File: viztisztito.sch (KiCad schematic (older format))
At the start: 0 parts

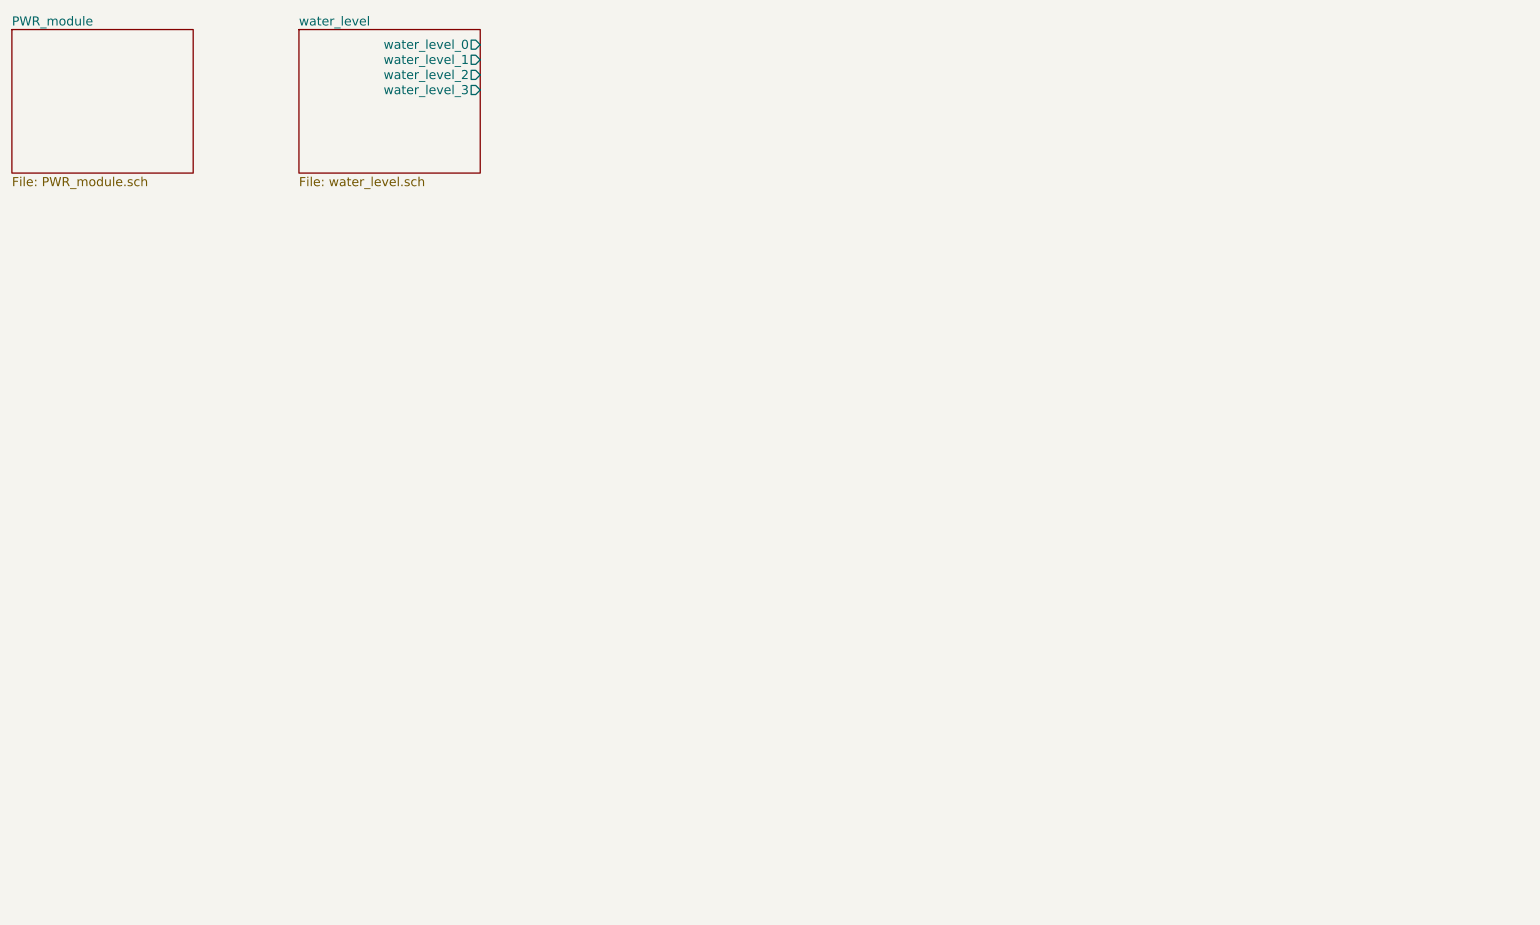
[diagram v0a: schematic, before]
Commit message: sch almost ready
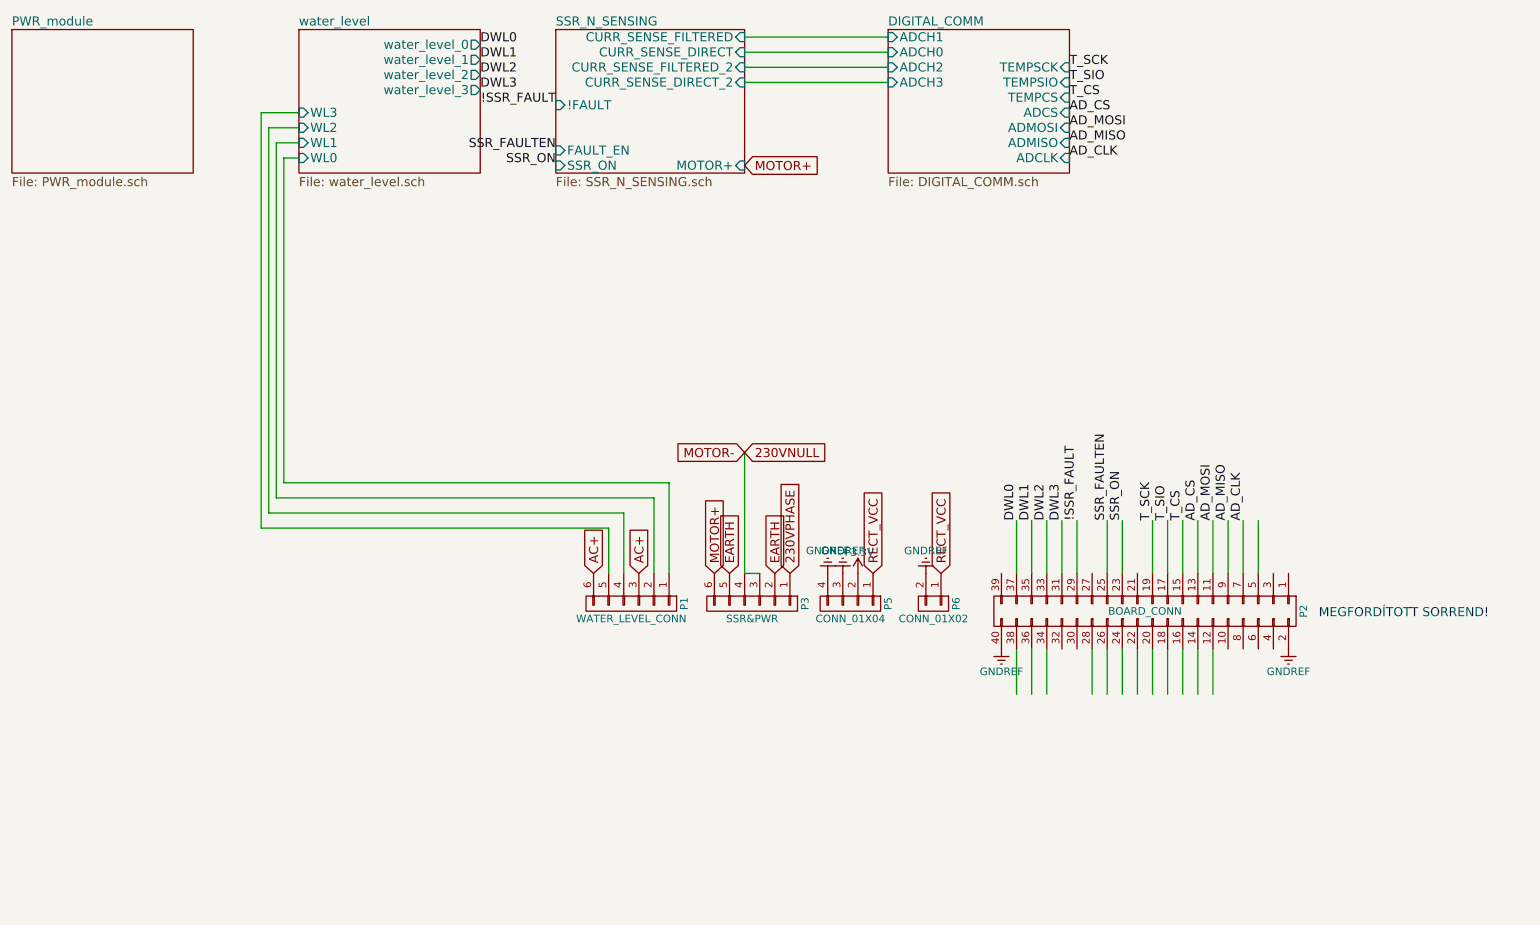
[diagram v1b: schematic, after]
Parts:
- added P1: WATER_LEVEL_CONN, symbol CONN_01X06
- added P2: BOARD_CONN, Socket_Strips:Socket_Strip_Straight_2x20, symbol CONN_02X20
- added P3: SSR&PWR, symbol CONN_01X06
- added P5: CONN_01X04, symbol CONN_01X04
- added P6: CONN_01X02, Pin_Headers:Pin_Header_Straight_1x02, symbol CONN_01X02
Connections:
- net labels added: !SSR_FAULT, +3.3V, 230VNULL, 230VPHASE, AC+, AD_CLK, AD_CS, AD_MISO, AD_MOSI, DWL0, DWL1, DWL2, DWL3, EARTH, GNDREF, MOTOR+, MOTOR-, RECT_VCC, SSR_FAULTEN, SSR_ON, T_CS, T_SCK, T_SIO
- wire segments 0 -> 49
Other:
- note added: "MEGFORDÍTOTT SORREND!"

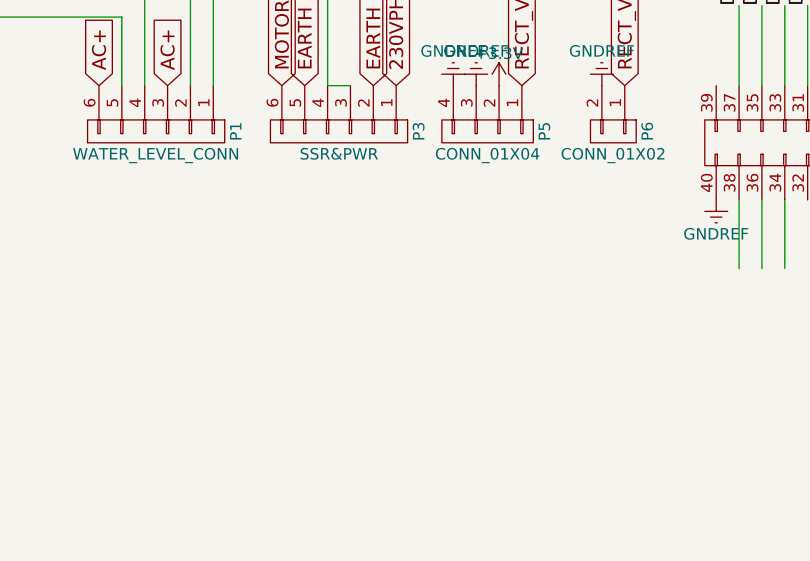
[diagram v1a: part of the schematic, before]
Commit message: sch ready, begining of layout
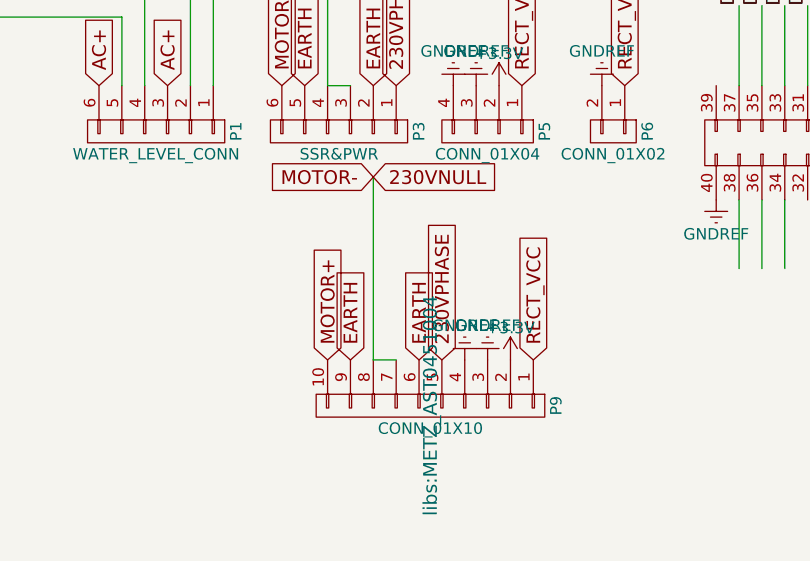
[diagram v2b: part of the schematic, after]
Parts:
- added P9: CONN_01X10, libs:METZ_AST0451004, symbol CONN_01X10
- P1, P3: footprint (none) -> libs:METZ_AST1350604
- P5: footprint (none) -> libs:METZ_AST1350404
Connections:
- wire segments 49 -> 51
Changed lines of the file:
@@
 F 0 "P1" H 5350 5150 50  0000 C CNN
 F 1 "WATER_LEVEL_CONN" V 5450 4800 50  0000 C CNN
-F 2 "" H 5350 4800 60  0001 C CNN
+F 2 "libs:METZ_AST1350604" H 5350 4800 60  0001 C CNN
 F 3 "" H 5350 4800 60  0000 C CNN
 	1    5350 4800
@@
 F 0 "P3" H 6150 5150 50  0000 C CNN
 F 1 "SSR&PWR" V 6250 4800 50  0000 C CNN
-F 2 "" H 6150 4800 60  0001 C CNN
+F 2 "libs:METZ_AST1350604" H 6150 4800 60  0001 C CNN
 F 3 "" H 6150 4800 60  0000 C CNN
 	1    6150 4800
@@
 F 0 "P5" H 6800 5050 50  0000 C CNN
 F 1 "CONN_01X04" V 6900 4800 50  0000 C CNN
-F 2 "" H 6800 4800 60  0001 C CNN
+F 2 "libs:METZ_AST1350404" H 6800 4800 60  0001 C CNN
 F 3 "" H 6800 4800 60  0000 C CNN
 	1    6800 4800
@@
 Wire Wire Line
 	6100 1350 7050 1350
+$Comp
+L CONN_01X10 P9
+U 1 1 5626D6E9
+P 6550 6000
+F 0 "P9" H 6550 6550 50  0000 C CNN
+F 1 "CONN_01X10" V 6650 6000 50  0000 C CNN
+F 2 "libs:METZ_AST0451004" H 6550 6000 60  0000 C CNN
+F 3 "" H 6550 6000 60  0000 C CNN
+	1    6550 6000
+	0    1    1    0
+$EndComp
+Text GLabel 7000 5800 1    60   Input ~ 0
+RECT_VCC
+$Comp
+L GNDREF #PWR07
+U 1 1 5626F098
+P 6700 5800
+F 0 "#PWR07" H 6700 5550 50  0001 C CNN
+F 1 "GNDREF" H 6700 5650 50  0000 C CNN
+F 2 "" H 6700 5800 60  0000 C CNN
+F 3 "" H 6700 5800 60  0000 C CNN
+	1    6700 5800
+	-1   0    0    1
+$EndComp
+$Comp
+L +3.3V #PWR08
+U 1 1 5626F09E
+P 6900 5800
+F 0 "#PWR08" H 6900 5650 50  0001 C CNN
+F 1 "+3.3V" H 6900 5940 50  0000 C CNN
+F 2 "" H 6900 5800 60  0000 C CNN
+F 3 "" H 6900 5800 60  0000 C CNN
+	1    6900 5800
+	1    0    0    -1
+$EndComp
+$Comp
+L GNDREF #PWR09
+U 1 1 5626F0A4
+P 6800 5800
+F 0 "#PWR09" H 6800 5550 50  0001 C CNN
+F 1 "GNDREF" H 6800 5650 50  0000 C CNN
+F 2 "" H 6800 5800 60  0000 C CNN
+F 3 "" H 6800 5800 60  0000 C CNN
+	1    6800 5800
+	-1   0    0    1
+$EndComp
+Text GLabel 6500 5800 1    60   Input ~ 0
+EARTH
+Text GLabel 6100 5800 1    60   Input ~ 0
+MOTOR+
+Text GLabel 6300 5000 0    60   Input ~ 0
+MOTOR-
+Text GLabel 6200 5800 1    60   Input ~ 0
+EARTH
+Wire Wire Line
+	6300 5000 6300 5800
+Wire Wire Line
+	6300 5800 6400 5800
+Text GLabel 6600 5800 1    60   Input ~ 0
+230VPHASE
+Text GLabel 6300 5000 2    60   Input ~ 0
+230VNULL
 $EndSCHEMATC

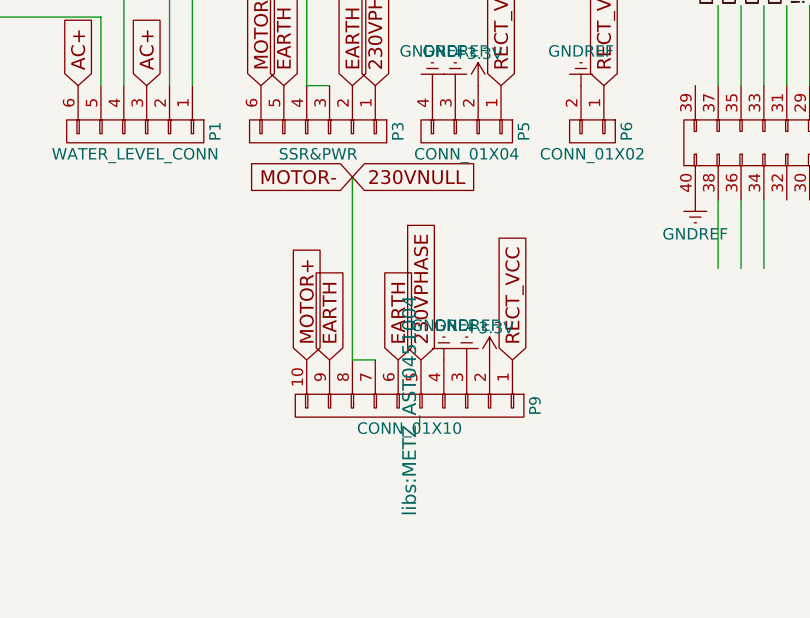
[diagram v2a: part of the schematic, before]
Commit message: layout beginning
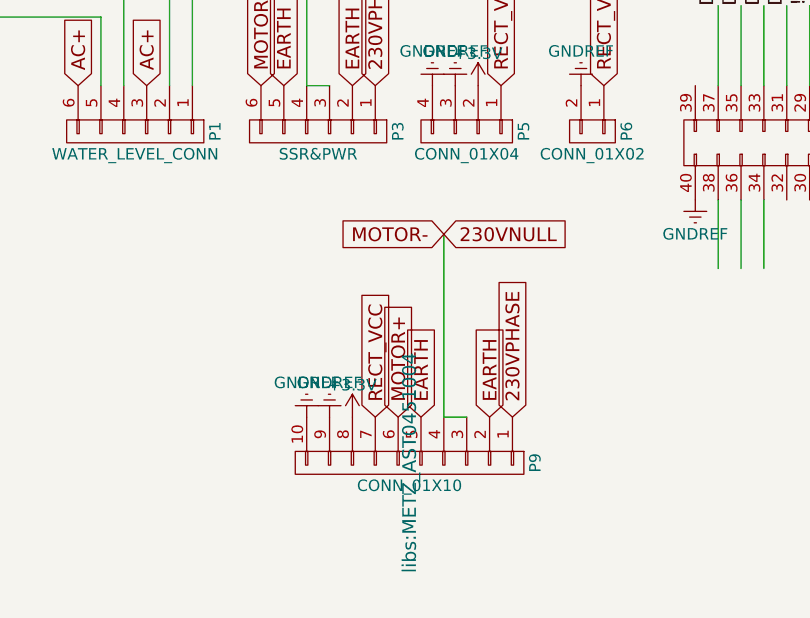
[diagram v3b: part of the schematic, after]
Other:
- moved on the sheet: P9
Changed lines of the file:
@@
 L CONN_01X10 P9
 U 1 1 5626D6E9
-P 6550 6000
-F 0 "P9" H 6550 6550 50  0000 C CNN
-F 1 "CONN_01X10" V 6650 6000 50  0000 C CNN
-F 2 "libs:METZ_AST0451004" H 6550 6000 60  0000 C CNN
-F 3 "" H 6550 6000 60  0000 C CNN
-	1    6550 6000
+P 6550 6250
+F 0 "P9" H 6550 6800 50  0000 C CNN
+F 1 "CONN_01X10" V 6650 6250 50  0000 C CNN
+F 2 "libs:METZ_AST0451004" H 6550 6250 60  0000 C CNN
+F 3 "" H 6550 6250 60  0000 C CNN
+	1    6550 6250
 	0    1    1    0
 $EndComp
-Text GLabel 7000 5800 1    60   Input ~ 0
+Text GLabel 6400 6050 1    60   Input ~ 0
 RECT_VCC
 $Comp
 L GNDREF #PWR07
 U 1 1 5626F098
-P 6700 5800
-F 0 "#PWR07" H 6700 5550 50  0001 C CNN
-F 1 "GNDREF" H 6700 5650 50  0000 C CNN
-F 2 "" H 6700 5800 60  0000 C CNN
-F 3 "" H 6700 5800 60  0000 C CNN
-	1    6700 5800
+P 6100 6050
+F 0 "#PWR07" H 6100 5800 50  0001 C CNN
+F 1 "GNDREF" H 6100 5900 50  0000 C CNN
+F 2 "" H 6100 6050 60  0000 C CNN
+F 3 "" H 6100 6050 60  0000 C CNN
+	1    6100 6050
 	-1   0    0    1
 $EndComp
@@
 L +3.3V #PWR08
 U 1 1 5626F09E
-P 6900 5800
-F 0 "#PWR08" H 6900 5650 50  0001 C CNN
-F 1 "+3.3V" H 6900 5940 50  0000 C CNN
-F 2 "" H 6900 5800 60  0000 C CNN
-F 3 "" H 6900 5800 60  0000 C CNN
-	1    6900 5800
+P 6300 6050
+F 0 "#PWR08" H 6300 5900 50  0001 C CNN
+F 1 "+3.3V" H 6300 6190 50  0000 C CNN
+F 2 "" H 6300 6050 60  0000 C CNN
+F 3 "" H 6300 6050 60  0000 C CNN
+	1    6300 6050
 	1    0    0    -1
 $EndComp
@@
 L GNDREF #PWR09
 U 1 1 5626F0A4
-P 6800 5800
-F 0 "#PWR09" H 6800 5550 50  0001 C CNN
-F 1 "GNDREF" H 6800 5650 50  0000 C CNN
-F 2 "" H 6800 5800 60  0000 C CNN
-F 3 "" H 6800 5800 60  0000 C CNN
-	1    6800 5800
+P 6200 6050
+F 0 "#PWR09" H 6200 5800 50  0001 C CNN
+F 1 "GNDREF" H 6200 5900 50  0000 C CNN
+F 2 "" H 6200 6050 60  0000 C CNN
+F 3 "" H 6200 6050 60  0000 C CNN
+	1    6200 6050
 	-1   0    0    1
 $EndComp
-Text GLabel 6500 5800 1    60   Input ~ 0
+Text GLabel 6900 6050 1    60   Input ~ 0
 EARTH
-Text GLabel 6100 5800 1    60   Input ~ 0
+Text GLabel 6500 6050 1    60   Input ~ 0
 MOTOR+
-Text GLabel 6300 5000 0    60   Input ~ 0
+Text GLabel 6700 5250 0    60   Input ~ 0
 MOTOR-
-Text GLabel 6200 5800 1    60   Input ~ 0
+Text GLabel 6600 6050 1    60   Input ~ 0
 EARTH
 Wire Wire Line
-	6300 5000 6300 5800
+	6700 5250 6700 6050
 Wire Wire Line
-	6300 5800 6400 5800
-Text GLabel 6600 5800 1    60   Input ~ 0
+	6700 6050 6800 6050
+Text GLabel 7000 6050 1    60   Input ~ 0
 230VPHASE
-Text GLabel 6300 5000 2    60   Input ~ 0
+Text GLabel 6700 5250 2    60   Input ~ 0
 230VNULL
 $EndSCHEMATC
